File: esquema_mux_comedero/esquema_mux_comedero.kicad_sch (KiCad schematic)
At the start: 3 parts

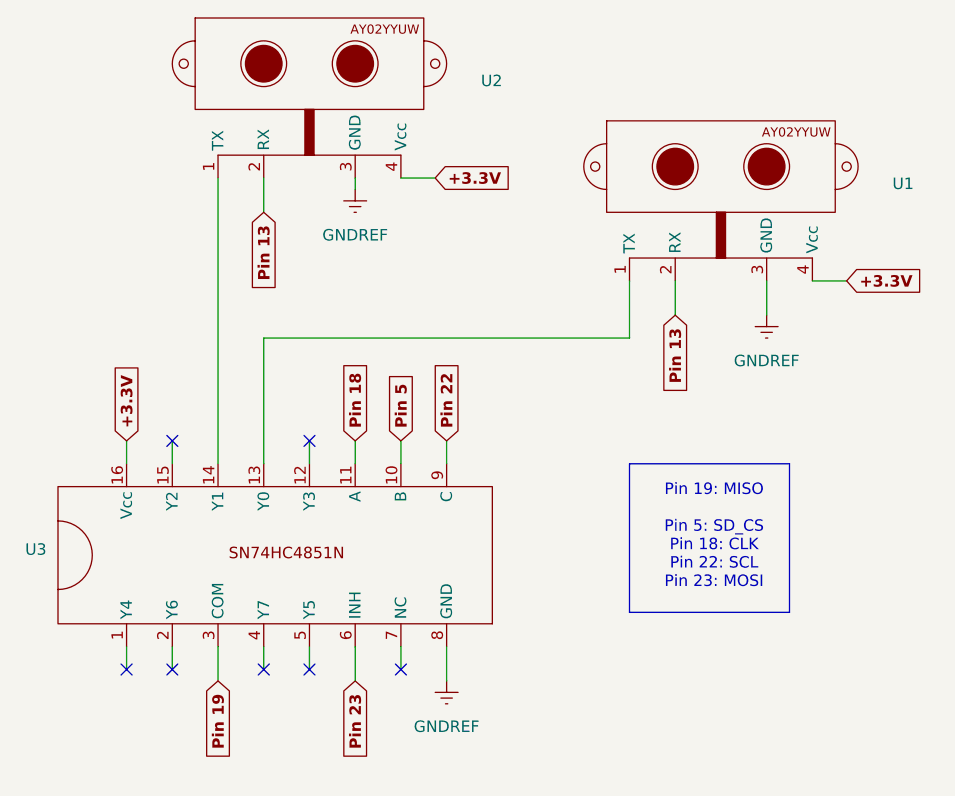
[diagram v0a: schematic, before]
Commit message: opr docu
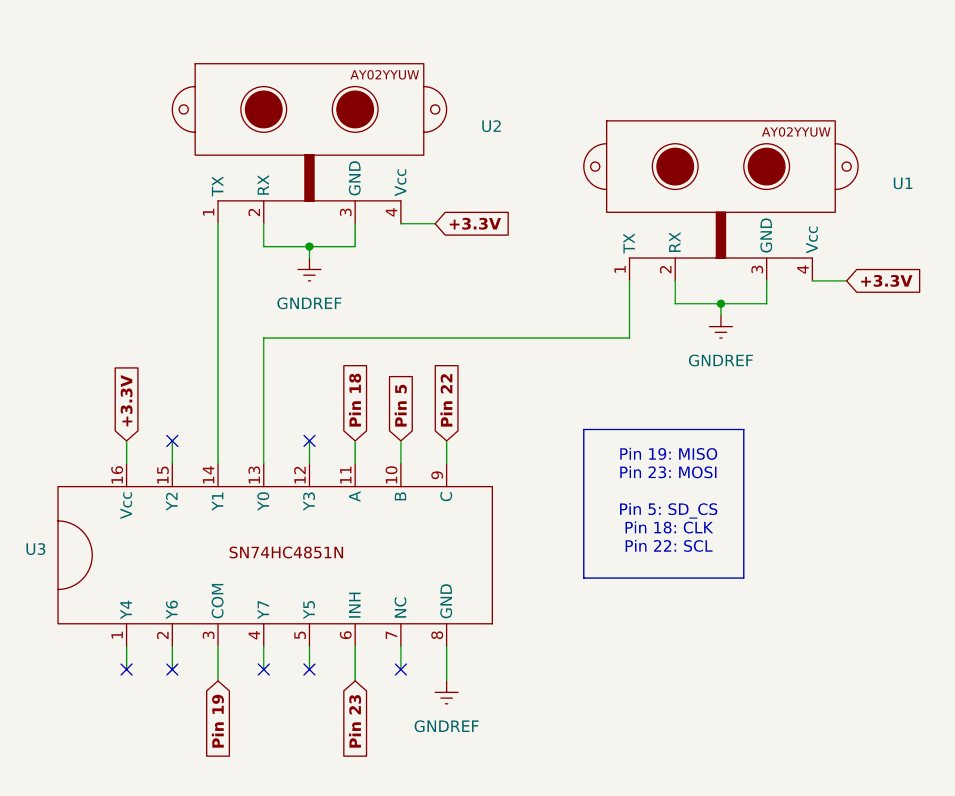
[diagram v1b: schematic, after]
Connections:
- net Pin 13 is gone; now on net GNDREF: U1.2 (RX), U2.2 (RX)
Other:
- note added: "Pin 19: MISO Pin 23: MOSI Pin 5: SD_CS Pin 18: CLK Pin 22: SCL"
- note removed: "Pin 19: MISO Pin 5: SD_CS Pin 18: CLK Pin 22: SCL Pin 23: MOSI"
- moved on the sheet: U2
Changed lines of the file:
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@@
 	(generator_version "8.0")
 	(paper "A4")
+	(junction
+		(at 106.68 102.87)
+		(diameter 0)
+		(color 0 0 0 0)
+	)
+	(junction
+		(at 152.4 109.22)
+		(diameter 0)
+		(color 0 0 0 0)
+	)
 	(no_connect
 		(at 86.36 149.86)
@@
 		)
 	)
+	(wire
+		(pts
+			(xy 111.76 102.87) (xy 111.76 100.33)
+		)
+		(stroke
+			(width 0)
+			(type default)
+		)
+	)
 	(bus
 		(pts
-			(xy 142.24 127) (xy 160.02 127)
+			(xy 137.16 123.19) (xy 154.94 123.19)
 		)
 		(stroke
@@
 	(bus
 		(pts
-			(xy 142.24 143.51) (xy 160.02 143.51)
+			(xy 137.16 139.7) (xy 154.94 139.7)
 		)
 		(stroke
@@
 	(bus
 		(pts
-			(xy 142.24 127) (xy 142.24 143.51)
+			(xy 137.16 123.19) (xy 137.16 139.7)
 		)
 		(stroke
@@
 	(wire
 		(pts
-			(xy 101.6 95.25) (xy 101.6 99.06)
+			(xy 101.6 100.33) (xy 101.6 102.87)
 		)
 		(stroke
@@
 	(wire
 		(pts
-			(xy 96.52 95.25) (xy 96.52 127)
+			(xy 96.52 100.33) (xy 96.52 127)
 		)
 		(stroke
@@
 	(wire
 		(pts
-			(xy 157.48 106.68) (xy 157.48 110.49)
+			(xy 152.4 109.22) (xy 152.4 110.49)
 		)
 		(stroke
@@
 	(wire
 		(pts
-			(xy 111.76 95.25) (xy 111.76 96.52)
+			(xy 152.4 109.22) (xy 157.48 109.22)
+		)
+		(stroke
+			(width 0)
+			(type default)
+		)
+	)
+	(wire
+		(pts
+			(xy 147.32 109.22) (xy 152.4 109.22)
 		)
 		(stroke
@@
 	(bus
 		(pts
-			(xy 160.02 143.51) (xy 160.02 127)
+			(xy 154.94 139.7) (xy 154.94 123.19)
 		)
 		(stroke
@@
 	(wire
 		(pts
-			(xy 116.84 95.25) (xy 120.65 95.25)
+			(xy 116.84 100.33) (xy 120.65 100.33)
+		)
+		(stroke
+			(width 0)
+			(type default)
+		)
+	)
+	(wire
+		(pts
+			(xy 101.6 102.87) (xy 106.68 102.87)
 		)
 		(stroke
@@
 	(wire
 		(pts
+			(xy 106.68 102.87) (xy 106.68 104.14)
+		)
+		(stroke
+			(width 0)
+			(type default)
+		)
+	)
+	(wire
+		(pts
 			(xy 101.6 149.86) (xy 101.6 147.32)
 		)
@@
 	(wire
 		(pts
-			(xy 147.32 106.68) (xy 147.32 110.49)
+			(xy 147.32 106.68) (xy 147.32 109.22)
+		)
+		(stroke
+			(width 0)
+			(type default)
+		)
+	)
+	(wire
+		(pts
+			(xy 106.68 102.87) (xy 111.76 102.87)
+		)
+		(stroke
+			(width 0)
+			(type default)
+		)
+	)
+	(wire
+		(pts
+			(xy 157.48 109.22) (xy 157.48 106.68)
 		)
 		(stroke
@@
 		)
 	)
-	(text "Pin 19: MISO\n\nPin 5: SD_CS\nPin 18: CLK\nPin 22: SCL\nPin 23: MOSI\n"
+	(text "Pin 19: MISO\nPin 23: MOSI\n\nPin 5: SD_CS\nPin 18: CLK\nPin 22: SCL\n"
 		(exclude_from_sim no)
-		(at 151.638 135.128 0)
+		(at 146.558 131.318 0)
 		(effects
 			(font
@@
 		)
 	)
-	(global_label "Pin 13"
+	(global_label "+3.3V"
 		(shape input)
-		(at 101.6 99.06 270)
+		(at 120.65 100.33 0)
 		(fields_autoplaced yes)
 		(effects
@@
 				(thickness 0.254)
 				(bold yes)
-				(color 221 133 0 1)
-			)
-			(justify right)
+			)
+			(justify left)
 		)
 		(property "Intersheetrefs" "${INTERSHEET_REFS}"
-			(at 101.6 108.9316 90)
-			(effects
-				(font
-					(size 1.27 1.27)
-				)
-				(justify right)
-				(hide yes)
-			)
-		)
-	)
-	(global_label "+3.3V"
-		(shape input)
-		(at 120.65 95.25 0)
-		(fields_autoplaced yes)
-		(effects
-			(font
-				(size 1.27 1.27)
-				(thickness 0.254)
-				(bold yes)
-			)
-			(justify left)
-		)
-		(property "Intersheetrefs" "${INTERSHEET_REFS}"
-			(at 129.796 95.25 0)
+			(at 129.796 100.33 0)
 			(effects
 				(font
@@
 		)
 	)
-	(global_label "Pin 13"
+	(global_label "+3.3V"
 		(shape input)
-		(at 147.32 110.49 270)
+		(at 86.36 124.46 90)
 		(fields_autoplaced yes)
 		(effects
@@
 				(thickness 0.254)
 				(bold yes)
-				(color 221 133 0 1)
-			)
-			(justify right)
-		)
-		(property "Intersheetrefs" "${INTERSHEET_REFS}"
-			(at 147.32 120.3616 90)
-			(effects
-				(font
-					(size 1.27 1.27)
-				)
-				(justify right)
-				(hide yes)
-			)
-		)
-	)
-	(global_label "+3.3V"
-		(shape input)
-		(at 86.36 124.46 90)
-		(fields_autoplaced yes)
-		(effects
-			(font
-				(size 1.27 1.27)
-				(thickness 0.254)
-				(bold yes)
 			)
 			(justify left)
@@
 	(symbol
 		(lib_id "power:GNDREF")
-		(at 157.48 110.49 0)
+		(at 152.4 110.49 0)
 		(unit 1)
 		(exclude_from_sim no)
@@
 		(fields_autoplaced yes)
 		(property "Reference" "#PWR01"
-			(at 157.48 116.84 0)
+			(at 152.4 116.84 0)
 			(effects
 				(font
@@
 		)
 		(property "Value" "GNDREF"
-			(at 157.48 115.57 0)
+			(at 152.4 115.57 0)
 			(effects
 				(font
@@
 		)
 		(property "Footprint" ""
-			(at 157.48 110.49 0)
+			(at 152.4 110.49 0)
 			(effects
 				(font
@@
 		)
 		(property "Datasheet" ""
-			(at 157.48 110.49 0)
+			(at 152.4 110.49 0)
 			(effects
 				(font
@@
 		)
 		(property "Description" "Power symbol creates a global label with name \"GNDREF\" , reference supply ground"
-			(at 157.48 110.49 0)
+			(at 152.4 110.49 0)
 			(effects
 				(font
@@
 	(symbol
 		(lib_id "power:GNDREF")
-		(at 111.76 96.52 0)
+		(at 106.68 104.14 0)
 		(unit 1)
 		(exclude_from_sim no)
@@
 		(fields_autoplaced yes)
 		(property "Reference" "#PWR04"
-			(at 111.76 102.87 0)
+			(at 106.68 110.49 0)
 			(effects
 				(font
@@
 		)
 		(property "Value" "GNDREF"
-			(at 111.76 101.6 0)
+			(at 106.68 109.22 0)
 			(effects
 				(font
@@
 		)
 		(property "Footprint" ""
-			(at 111.76 96.52 0)
+			(at 106.68 104.14 0)
 			(effects
 				(font
@@
 		)
 		(property "Datasheet" ""
-			(at 111.76 96.52 0)
+			(at 106.68 104.14 0)
 			(effects
 				(font
@@
 		)
 		(property "Description" "Power symbol creates a global label with name \"GNDREF\" , reference supply ground"
-			(at 111.76 96.52 0)
+			(at 106.68 104.14 0)
 			(effects
 				(font
@@
 		(lib_name "A02YYUW_1")
 		(lib_id "Mensoft_Carmen:A02YYUW")
-		(at 106.68 82.55 0)
+		(at 106.68 87.63 0)
 		(unit 1)
 		(exclude_from_sim no)
@@
 		(fields_autoplaced yes)
 		(property "Reference" "U2"
-			(at 125.73 84.4549 0)
+			(at 125.73 89.5349 0)
 			(effects
 				(font
@@
 		)
 		(property "Value" "~"
-			(at 125.73 86.36 0)
+			(at 125.73 91.44 0)
 			(effects
 				(font
@@
 		)
 		(property "Footprint" ""
-			(at 106.68 82.55 0)
+			(at 106.68 87.63 0)
 			(effects
 				(font
@@
 		)
 		(property "Datasheet" ""
-			(at 106.68 82.55 0)
+			(at 106.68 87.63 0)
 			(effects
 				(font
@@
 		)
 		(property "Description" ""
-			(at 106.68 82.55 0)
-			(effects
-				(font
+			(at 106.68 87.63 0)
+			(effects
+				(font
